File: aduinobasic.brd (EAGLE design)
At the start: 111.8 x 60.6 mm, 108 parts, among them SW1 POW

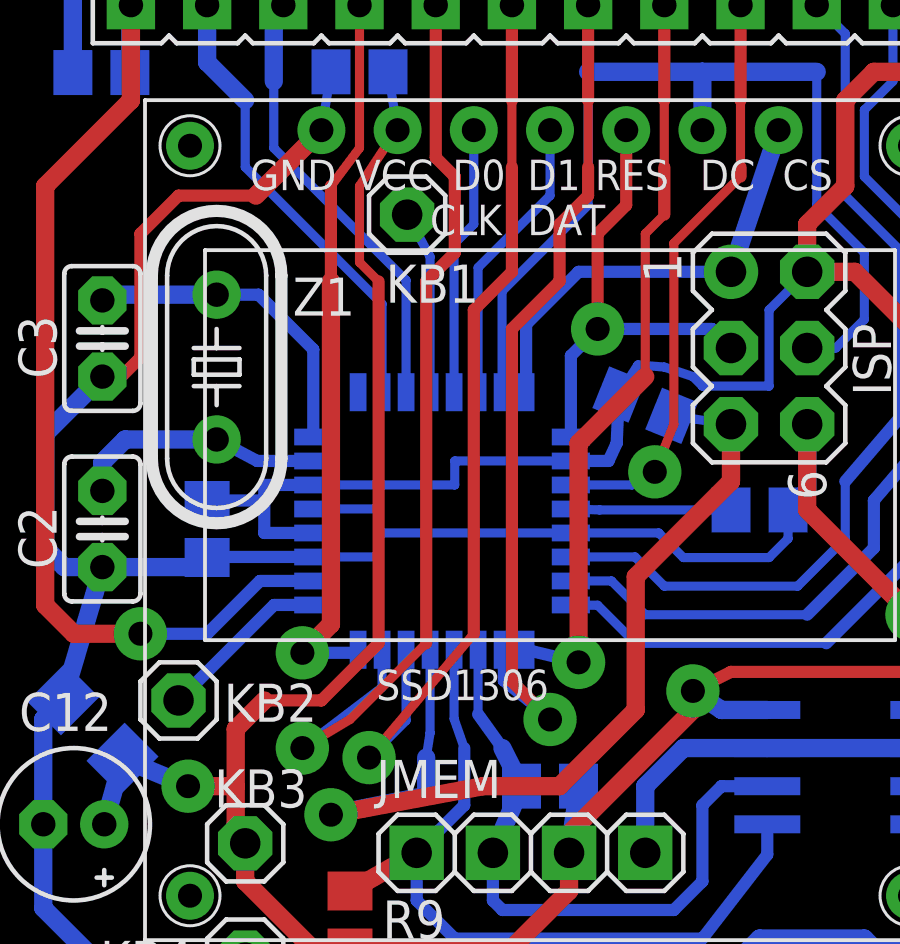
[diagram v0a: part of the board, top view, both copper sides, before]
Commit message: .
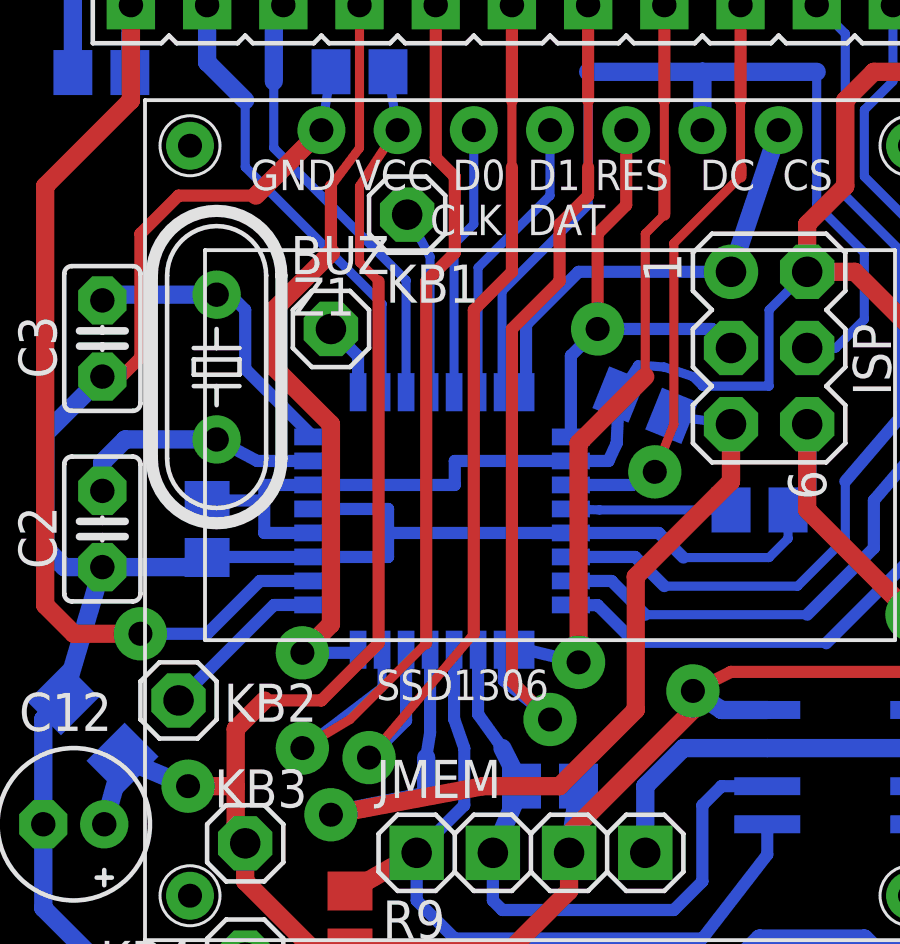
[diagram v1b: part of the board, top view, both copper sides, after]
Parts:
- added BUZ: (no value), pinhead:1X01
- VT1, VT2, VT3: value (none) -> КТ315Б
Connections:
- net BUZ: now also BUZ.1
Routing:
- net BUZ: track 0.00 -> 2.48 mm
- net D2: track 24.2 -> 25.8 mm
- net N$2: track 10.8 -> 10.2 mm

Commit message: .
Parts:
- R11: value 180 -> 200
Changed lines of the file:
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@@
 <attribute name="VALUE" x="83.5025" y="53.5305" size="1.27" layer="28" rot="MR0"/>
 </element>
-<element name="R11" library="rcl" package="M1206" value="180" x="64.4525" y="57.785" smashed="yes" rot="MR270">
+<element name="R11" library="rcl" package="M1206" value="200" x="64.4525" y="57.785" smashed="yes" rot="MR270">
 <attribute name="NAME" x="66.9925" y="59.055" size="1.27" layer="26" rot="MR270"/>
 <attribute name="VALUE" x="66.9925" y="59.055" size="1.27" layer="28" rot="MR270"/>
